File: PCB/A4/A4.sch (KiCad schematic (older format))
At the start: 39 parts, among them J1 Barrel_Jack_Switch, J13 Conn_01x06_Male, J15 Conn_01x06_Male, J2 Conn_01x02_Male, J25 Conn_01x04_Male, J3 Conn_01x06_Male, J4 Conn_01x02_Male, J7 Screw_Terminal_01x02, J8 Screw_Terminal_01x02, Q1 2N7002, Q2 2N7002, Q3 2N7002, Q4 2N7002, U1 AZ1117-3.3, U2 TB67H451FNG,EL, U3 ESP32-S2-WROOM, U4 TB67H451FNG,EL, U5 AZ1117-5.0

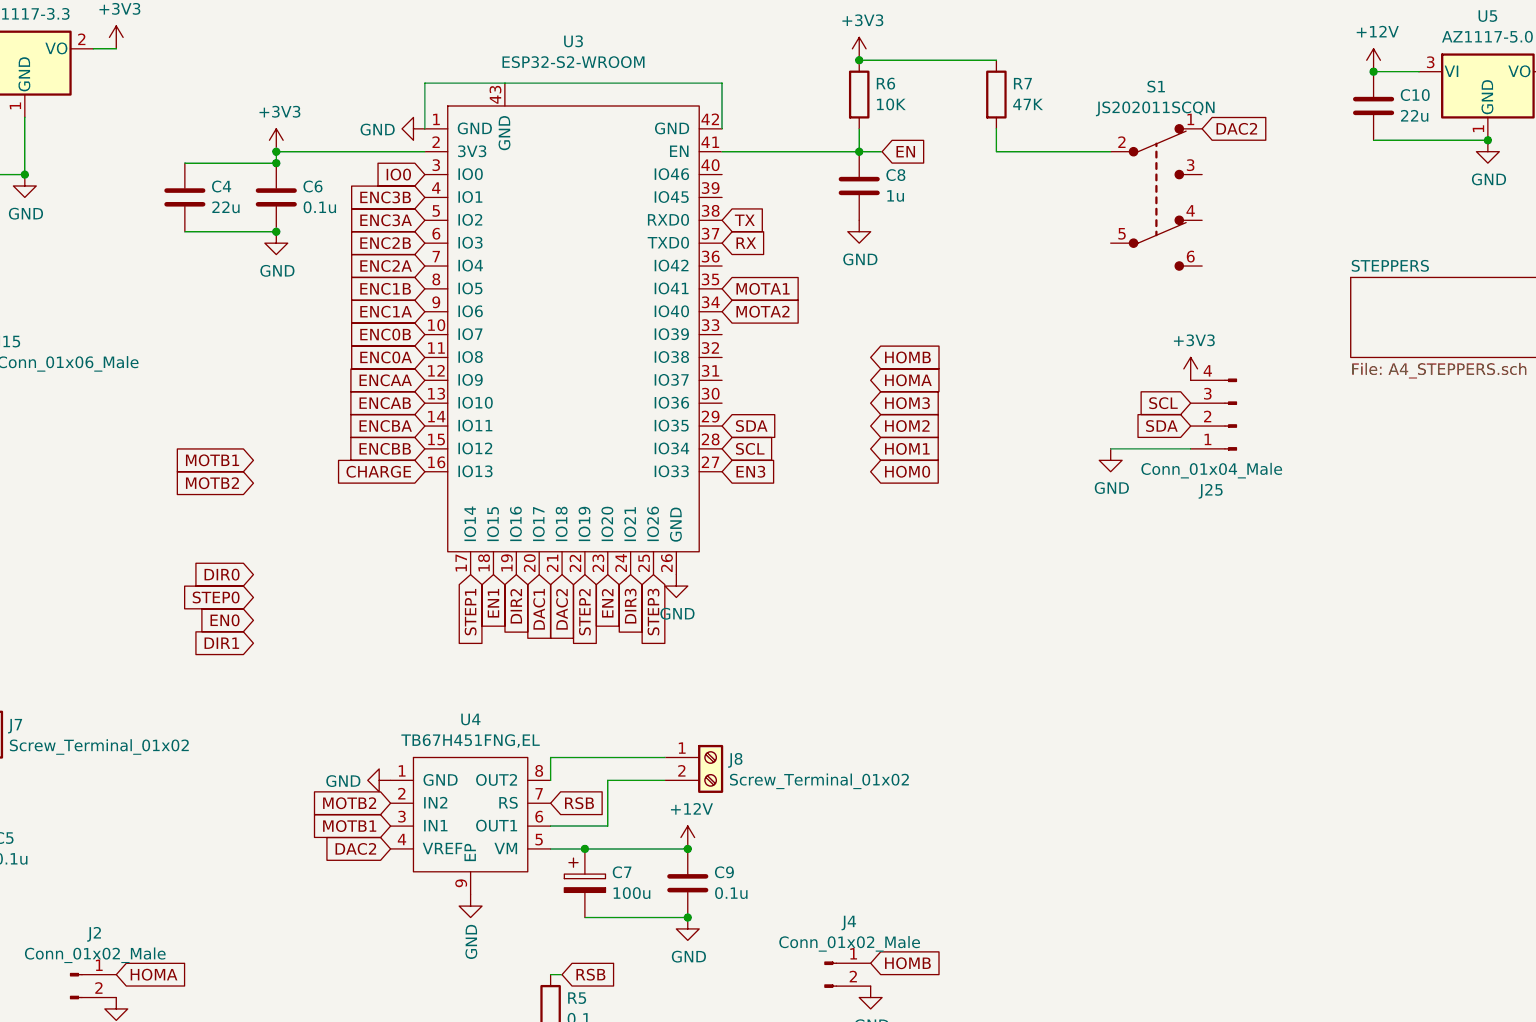
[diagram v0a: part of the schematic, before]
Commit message: PCB ready to order
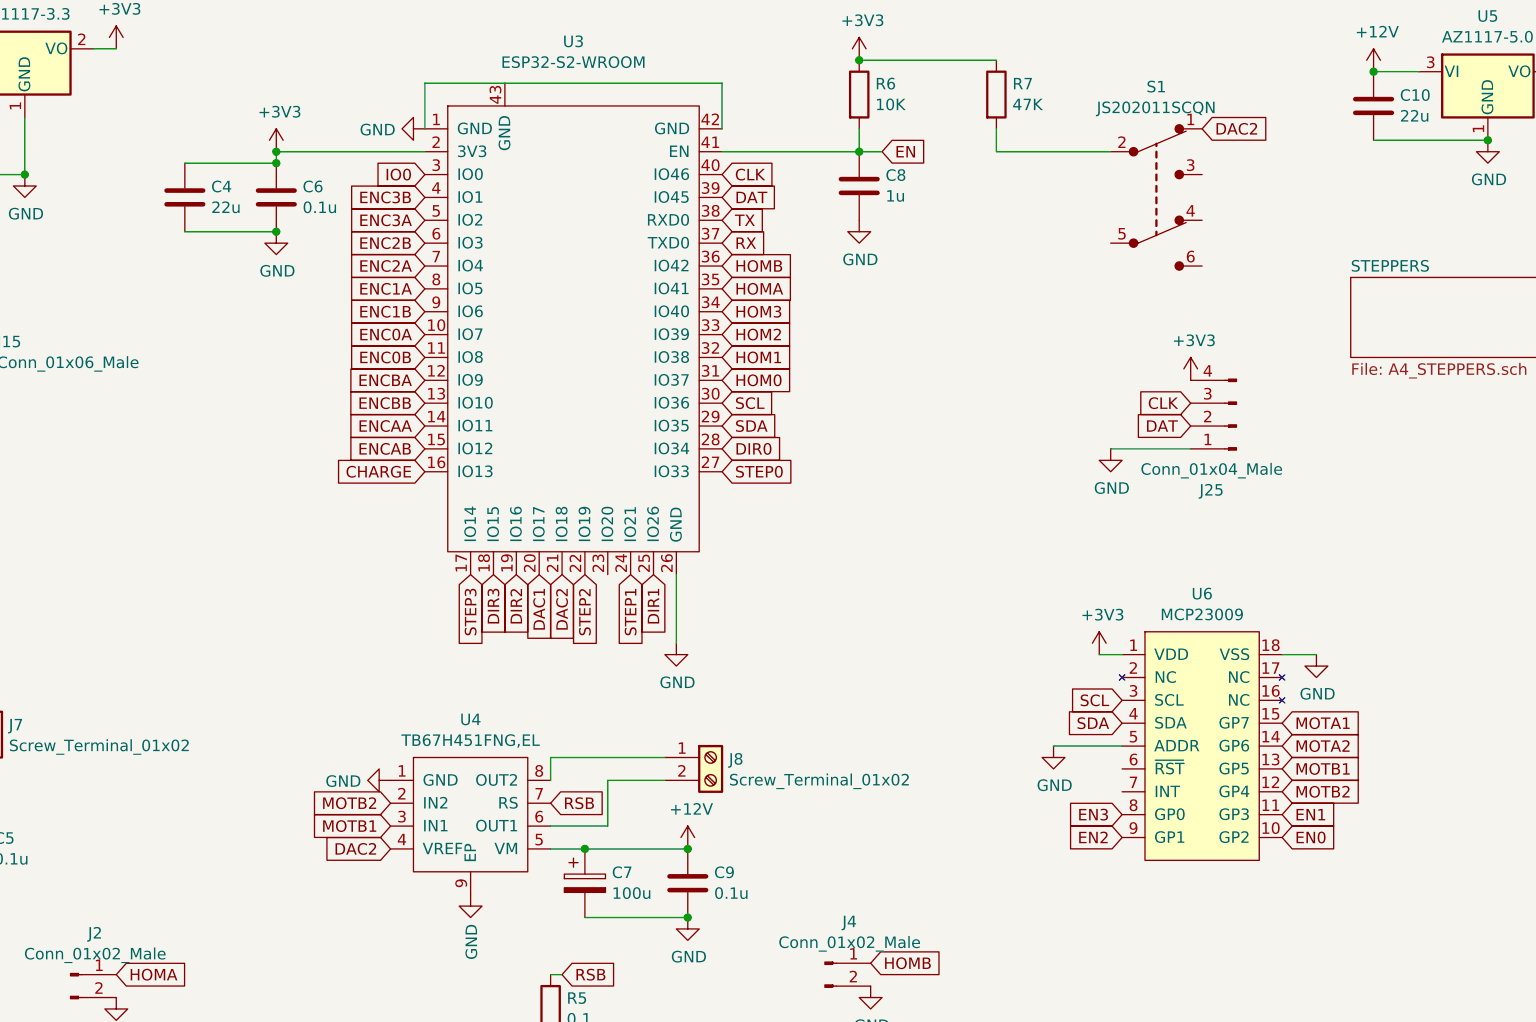
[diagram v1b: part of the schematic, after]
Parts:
- added U6: MCP23009, Package_SO:SOIC-18W_7.5x11.6mm_P1.27mm, symbol A4:MCP23009
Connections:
- net +3V3: now also U6.1 (VDD)
- net DIR0: now also U3.28 (IO34)
- net DIR1: now also U3.25 (IO26)
- net DIR3: now also U3.18 (IO15); no longer U3.24 (IO21)
- net EN0: now also U6.10 (GP2)
- net EN1: now also U6.11 (GP3); no longer U3.18 (IO15)
- net EN2: now also U6.9 (GP1); no longer U3.23 (IO20)
- net EN3: now also U6.8 (GP0); no longer U3.27 (IO33)
- net ENC0A: now also U3.10 (IO7); no longer U3.11 (IO8)
- net ENC0B: now also U3.11 (IO8); no longer U3.10 (IO7)
- net ENC1A: now also U3.8 (IO5); no longer U3.9 (IO6)
- net ENC1B: now also U3.9 (IO6); no longer U3.8 (IO5)
- net ENCAA: now also U3.14 (IO11); no longer U3.12 (IO9)
- net ENCAB: now also U3.15 (IO12); no longer U3.13 (IO10)
- net ENCBA: now also U3.12 (IO9); no longer U3.14 (IO11)
- net ENCBB: now also U3.13 (IO10); no longer U3.15 (IO12)
- net GND: now also U6.18 (VSS), U6.5 (ADDR)
- net HOM0: now also U3.31 (IO37)
- net HOM1: now also U3.32 (IO38)
- net HOM2: now also U3.33 (IO39)
- net HOM3: now also U3.34 (IO40)
- net HOMA: now also U3.35 (IO41)
- net HOMB: now also U3.36 (IO42)
- net MOTA1: now also U6.15 (GP7); no longer U3.35 (IO41)
- net MOTA2: now also U6.14 (GP6); no longer U3.34 (IO40)
- net MOTB1: now also U6.13 (GP5)
- net MOTB2: now also U6.12 (GP4)
- net SCL: now also U3.30 (IO36), U6.3 (SCL); no longer J25.3 (Pin_3), U3.28 (IO34)
- net SDA: now also U6.4 (SDA); no longer J25.2 (Pin_2)
- net STEP0: now also U3.27 (IO33)
- net STEP1: now also U3.24 (IO21); no longer U3.17 (IO14)
- net STEP3: now also U3.17 (IO14); no longer U3.25 (IO26)
- net DAT: now reaches U3.39 (IO45)
- net DAT: now also J25.2 (Pin_2)
- net CLK: now reaches U3.40 (IO46)
- net CLK: now also J25.3 (Pin_3)
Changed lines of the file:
@@
 L power:GND #PWR026
 U 1 1 60899FEA
-P 5650 3150
-F 0 "#PWR026" H 5650 2900 50  0001 C CNN
-F 1 "GND" H 5655 2977 50  0000 C CNN
-F 2 "" H 5650 3150 50  0001 C CNN
-F 3 "" H 5650 3150 50  0001 C CNN
-	1    5650 3150
+P 5650 3450
+F 0 "#PWR026" H 5650 3200 50  0001 C CNN
+F 1 "GND" H 5655 3277 50  0000 C CNN
+F 2 "" H 5650 3450 50  0001 C CNN
+F 3 "" H 5650 3450 50  0001 C CNN
+	1    5650 3450
 	1    0    0    -1
 $EndComp
@@
 Text GLabel 4550 2700 0    50   Input ~ 0
 CHARGE
-Text GLabel 4550 2400 0    50   Input ~ 0
+Text GLabel 4550 2600 0    50   Input ~ 0
 ENCAB
-Text GLabel 4550 2300 0    50   Input ~ 0
+Text GLabel 4550 2500 0    50   Input ~ 0
 ENCAA
 Wire Wire Line
@@
 	0    1    1    0
 $EndComp
-Text GLabel 5850 2000 2    50   Input ~ 0
+Text GLabel 8300 3900 2    50   Input ~ 0
 MOTA2
-Text GLabel 5850 1900 2    50   Input ~ 0
+Text GLabel 8300 3800 2    50   Input ~ 0
 MOTA1
 Text GLabel 1250 4100 0    50   Input ~ 0
@@
 Wire Wire Line
 	1100 5850 1650 5850
-Text GLabel 3800 3350 0    50   Input ~ 0
+Text GLabel 8300 4300 2    50   Input ~ 0
 EN0
-Text GLabel 3800 3250 0    50   Input ~ 0
+Text GLabel 5850 2700 2    50   Input ~ 0
 STEP0
-Text GLabel 3800 3150 0    50   Input ~ 0
+Text GLabel 5850 2600 2    50   Input ~ 0
 DIR0
 Wire Wire Line
@@
 Wire Wire Line
 	750  800  650  800
-Text GLabel 3800 2650 0    50   Input ~ 0
+Text GLabel 8300 4000 2    50   Input ~ 0
 MOTB1
-Text GLabel 3800 2750 0    50   Input ~ 0
+Text GLabel 8300 4100 2    50   Input ~ 0
 MOTB2
-Text GLabel 4550 2500 0    50   Input ~ 0
+Text GLabel 4550 2300 0    50   Input ~ 0
 ENCBA
-Text GLabel 4550 2600 0    50   Input ~ 0
+Text GLabel 4550 2400 0    50   Input ~ 0
 ENCBB
 Text GLabel 7950 1200 2    50   Input ~ 0
@@
 	1    0    0    -1
 $EndComp
-Text GLabel 3800 3450 0    50   Input ~ 0
+Text GLabel 5550 3150 3    50   Input ~ 0
 DIR1
-Text GLabel 4750 3150 3    50   Input ~ 0
+Text GLabel 5450 3150 3    50   Input ~ 0
 STEP1
-Text GLabel 4850 3150 3    50   Input ~ 0
+Text GLabel 8300 4200 2    50   Input ~ 0
 EN1
 Text GLabel 4950 3150 3    50   Input ~ 0
@@
 Text GLabel 5250 3150 3    50   Input ~ 0
 STEP2
-Text GLabel 5350 3150 3    50   Input ~ 0
+Text GLabel 7600 4300 0    50   Input ~ 0
 EN2
-Text GLabel 5450 3150 3    50   Input ~ 0
+Text GLabel 4850 3150 3    50   Input ~ 0
 DIR3
-Text GLabel 5550 3150 3    50   Input ~ 0
+Text GLabel 4750 3150 3    50   Input ~ 0
 STEP3
-Text GLabel 5850 2700 2    50   Input ~ 0
+Text GLabel 7600 4200 0    50   Input ~ 0
 EN3
 $Comp
@@
 F1 "A4_STEPPERS.sch" 50
 $EndSheet
-Text GLabel 6500 2700 2    50   Input ~ 0
+Text GLabel 5850 2300 2    50   Input ~ 0
 HOM0
-Text GLabel 6500 2600 2    50   Input ~ 0
+Text GLabel 5850 2200 2    50   Input ~ 0
 HOM1
-Text GLabel 6500 2500 2    50   Input ~ 0
+Text GLabel 5850 2100 2    50   Input ~ 0
 HOM2
-Text GLabel 6500 2400 2    50   Input ~ 0
+Text GLabel 5850 2000 2    50   Input ~ 0
 HOM3
-Text GLabel 6500 2300 2    50   Input ~ 0
+Text GLabel 5850 1900 2    50   Input ~ 0
 HOMA
-Text GLabel 6500 2200 2    50   Input ~ 0
+Text GLabel 5850 1800 2    50   Input ~ 0
 HOMB
 $Comp
@@
 Text GLabel 4550 1800 0    50   Input ~ 0
 ENC2A
+Text GLabel 4550 2000 0    50   Input ~ 0
+ENC1B
 Text GLabel 4550 1900 0    50   Input ~ 0
-ENC1B
-Text GLabel 4550 2000 0    50   Input ~ 0
 ENC1A
+Text GLabel 4550 2200 0    50   Input ~ 0
+ENC0B
 Text GLabel 4550 2100 0    50   Input ~ 0
-ENC0B
-Text GLabel 4550 2200 0    50   Input ~ 0
 ENC0A
 $Comp
@@
 Wire Wire Line
 	7550 2600 7900 2600
-Text GLabel 7900 2400 0    50   Input ~ 0
+Text GLabel 7600 3700 0    50   Input ~ 0
 SCL
-Text GLabel 7900 2500 0    50   Input ~ 0
+Text GLabel 7600 3800 0    50   Input ~ 0
 SDA
-Text GLabel 5850 2600 2    50   Input ~ 0
+Text GLabel 5850 2400 2    50   Input ~ 0
 SCL
 Text GLabel 5850 2500 2    50   Input ~ 0
 SDA
+$Comp
+L A4:MCP23009 U6
+U 1 1 608B6769
+P 7950 3900
+F 0 "U6" H 7950 4565 50  0000 C CNN
+F 1 "MCP23009" H 7950 4474 50  0000 C CNN
+F 2 "Package_SO:SOIC-18W_7.5x11.6mm_P1.27mm" H 7950 3950 50  0001 C CNN
+F 3 "" H 7950 3950 50  0001 C CNN
+	1    7950 3900
+	1    0    0    -1
+$EndComp
+Text GLabel 7900 2400 0    50   Input ~ 0
+CLK
+Text GLabel 7900 2500 0    50   Input ~ 0
+DAT
+$Comp
+L power:+3V3 #PWR0101
+U 1 1 608B8028
+P 7500 3500
+F 0 "#PWR0101" H 7500 3350 50  0001 C CNN
+F 1 "+3V3" H 7515 3673 50  0000 C CNN
+F 2 "" H 7500 3500 50  0001 C CNN
+F 3 "" H 7500 3500 50  0001 C CNN
+	1    7500 3500
+	1    0    0    -1
+$EndComp
+Wire Wire Line
+	7500 3500 7600 3500
+$Comp
+L power:GND #PWR0104
+U 1 1 608BAFEB
+P 7300 3900
+F 0 "#PWR0104" H 7300 3650 50  0001 C CNN
+F 1 "GND" H 7305 3727 50  0000 C CNN
+F 2 "" H 7300 3900 50  0001 C CNN
+F 3 "" H 7300 3900 50  0001 C CNN
+	1    7300 3900
+	1    0    0    -1
+$EndComp
+Wire Wire Line
+	7300 3900 7600 3900
+$Comp
+L power:GND #PWR0108
+U 1 1 608BDF3C
+P 8450 3500
+F 0 "#PWR0108" H 8450 3250 50  0001 C CNN
+F 1 "GND" H 8455 3327 50  0000 C CNN
+F 2 "" H 8450 3500 50  0001 C CNN
+F 3 "" H 8450 3500 50  0001 C CNN
+	1    8450 3500
+	1    0    0    -1
+$EndComp
+Wire Wire Line
+	8300 3500 8450 3500
+Text GLabel 5850 1500 2    50   Input ~ 0
+DAT
+Text GLabel 5850 1400 2    50   Input ~ 0
+CLK
+Wire Wire Line
+	5650 3150 5650 3450
 $EndSCHEMATC
